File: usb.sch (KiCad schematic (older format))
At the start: 34 parts, among them IC1 EP4CE10F17, P1 USB_A, U23 FT313HL-LQFP64-0.5, U25 TPS2024D, Y2 12MHz

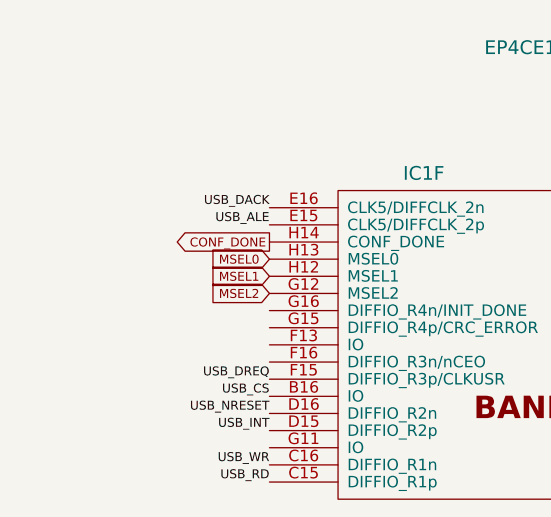
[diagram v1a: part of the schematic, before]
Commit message: A bit of update
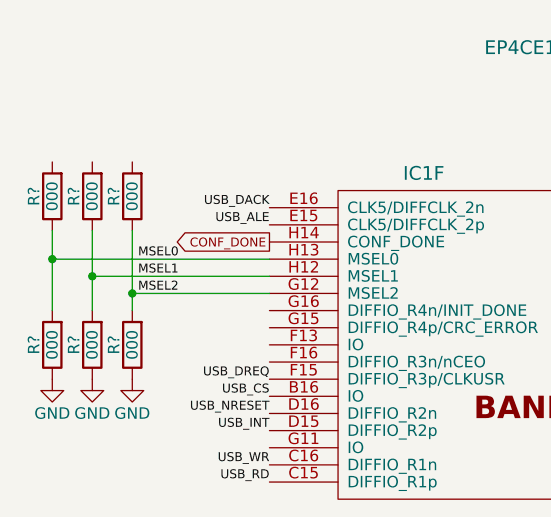
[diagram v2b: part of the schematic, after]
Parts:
- added R? (x6): 000, Resistors_SMD:R_0603, symbol R
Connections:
- net GND: now also R?.1, R?.1, R?.1
- net MSEL0: now also R?.1, R?.2
- net MSEL1: now also R?.1, R?.2
- net MSEL2: now also R?.1, R?.2
